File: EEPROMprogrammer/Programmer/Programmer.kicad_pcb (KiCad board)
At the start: 2 copper layers, 58.4 x 47 mm, 4 parts, among them U1 74HC595, U2 74HC595, U3 AT28C256B15PU

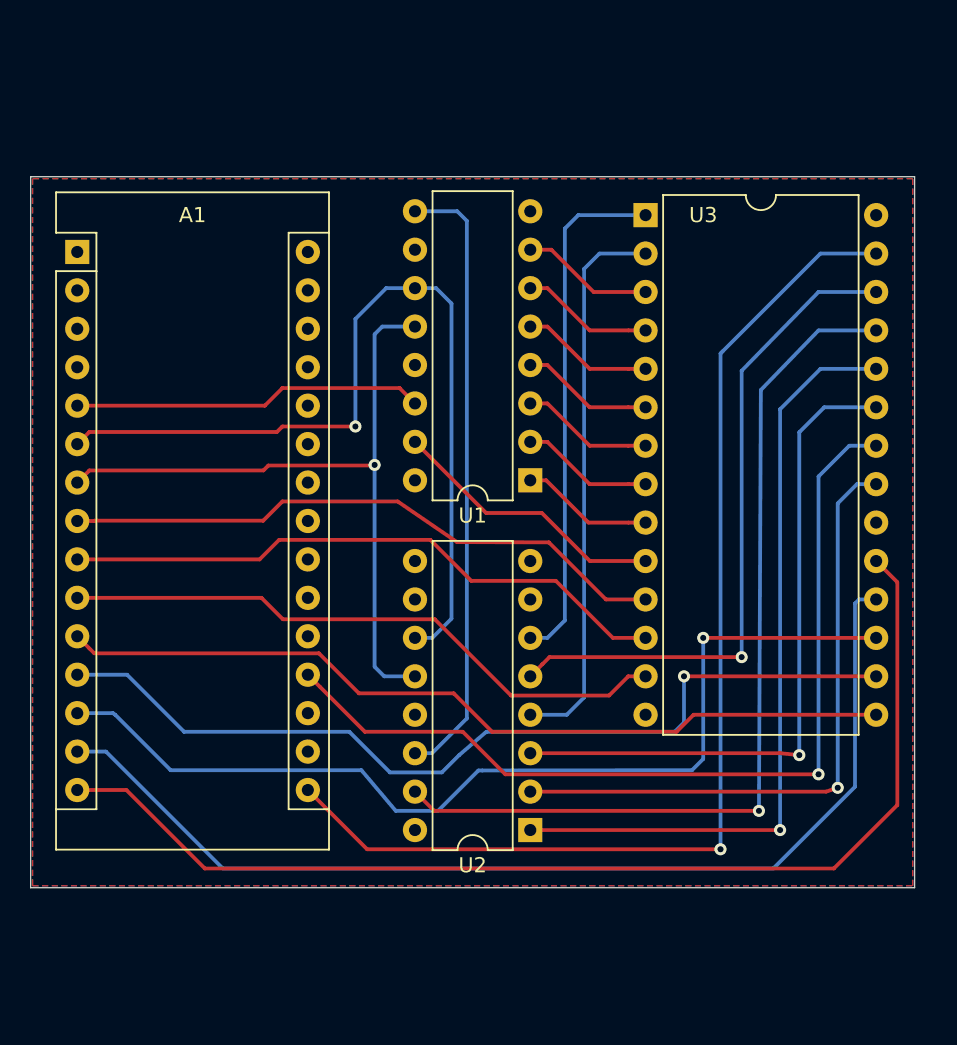
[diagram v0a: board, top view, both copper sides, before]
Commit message: In situ programming hw
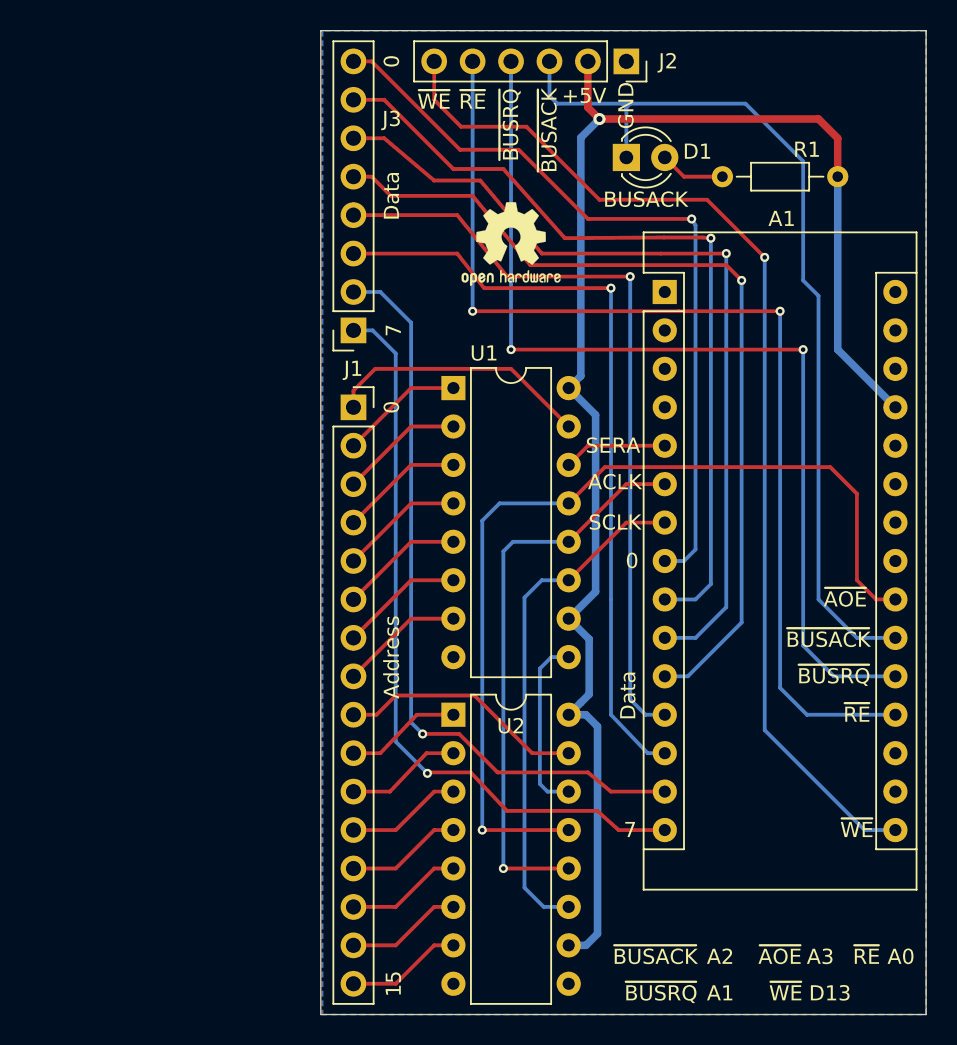
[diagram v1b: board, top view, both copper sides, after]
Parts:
- removed U3: AT28C256B15PU, Package_DIP:DIP-28_W15.24mm
- added D1: LED, LED_THT:LED_D3.0mm, F.Cu at (132.1, 67.3)
- added J1: Conn_01x16_Female, Connector_PinSocket_2.54mm:PinSocket_1x16_P2.54mm_Vertical, F.Cu at (114.0, 83.8)
- added J2: Conn_01x06_Female, Connector_PinSocket_2.54mm:PinSocket_1x06_P2.54mm_Vertical, F.Cu at (132.1, 61.0)
- added J3: Conn_01x08_Female, Connector_PinSocket_2.54mm:PinSocket_1x08_P2.54mm_Vertical, F.Cu at (114.0, 78.7)
- added R1: 2k2, Resistor_THT:R_Axial_DIN0204_L3.6mm_D1.6mm_P7.62mm_Horizontal, F.Cu at (146.1, 68.6)
- added REF**: OSHW-Logo2_7.3x6mm_SilkScreen, Symbol:OSHW-Logo2_7.3x6mm_SilkScreen, F.Cu at (124.5, 73.0)
- moved A1 38.9 mm to (134.6, 76.2)
- moved U2 9.16 mm to (120.7, 104.1), turned to 0 degrees
- moved U1 7.94 mm to (120.7, 82.5), turned to 0 degrees
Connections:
- A1 pad 19: /~OE -> /~RE
- A1 pad 20: Net-(A1-Pad20) -> /~BUSRQ
- A1 pad 21: Net-(A1-Pad21) -> /~BUSACK
- A1 pad 22: Net-(A1-Pad22) -> /~AOE
- A1 pad 6: /SHIFTCLK -> /ADRCLK
- A1 pad 7: /ADRCLK -> /SHIFTCLK
- U1 pad 13: GND -> /~AOE
- U2 pad 13: GND -> /~AOE
- U2 pad 7: Net-(U2-Pad7) -> /A15
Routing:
- net +5V: track 0.00 -> 100.7 mm, vias 0 -> 1
- net /~RE: track 0.00 -> 70.1 mm, vias 0 -> 2
- net /~BUSRQ: track 0.00 -> 64.8 mm, vias 0 -> 2
- net /~AOE: track 0.00 -> 61.9 mm, vias 0 -> 1
- net /~OE: track 60.8 -> 0.00 mm, vias 1 -> 0
- net /~BUSACK: track 0.00 -> 60.6 mm
- net /A9: track 51.8 -> 7.69 mm, vias 1 -> 0
- net /A8: track 60.4 -> 16.3 mm, vias 1 -> 0
- net /A11: track 44.9 -> 7.66 mm, vias 1 -> 0
- net /A13: track 44.5 -> 7.66 mm, vias 1 -> 0
- net /A10: track 42.2 -> 7.69 mm, vias 1 -> 0
- net /A12: track 36.8 -> 7.66 mm
- net Net-(U1-Pad9): track 41.0 -> 12.0 mm
- net /A14: track 34.4 -> 7.66 mm
- net /D7: track 74.8 -> 49.2 mm, vias 0 -> 1
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- added copper zone on F.Cu, net GND
- removed copper zone on F.Cu, net +5V
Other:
- board size 58.4 x 47 mm -> 40 x 65 mm
- net class Default: via_dia 0.8 -> 0.6; via_drill 0.4 -> 0.3
- net class Power added: clearance 0.3, trace_width 0.5, via_dia 0.8, via_drill 0.4
- board text added: "+5V"
- board text added: "0"
- board text added: "15"
- board text added: "7"
- board text added: "A0"
- board text added: "A1"
- board text added: "A2"
- board text added: "A3"
- board text added: "ACLK"
- board text added: "Address"
- board text added: "BUSACK"
- board text added: "D13"
- board text added: "Data"
- board text added: "GND"
- board text added: "SCLK"
- board text added: "SERA"
- board text added: "~AOE"
- board text added: "~BUSACK"
- board text added: "~BUSRQ"
- board text added: "~RE"
- board text added: "~WE"
